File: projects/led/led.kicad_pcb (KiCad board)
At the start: 2 copper layers, 18.2 x 12.8 mm, 3 parts, among them J1 Conn_01x02_Pin

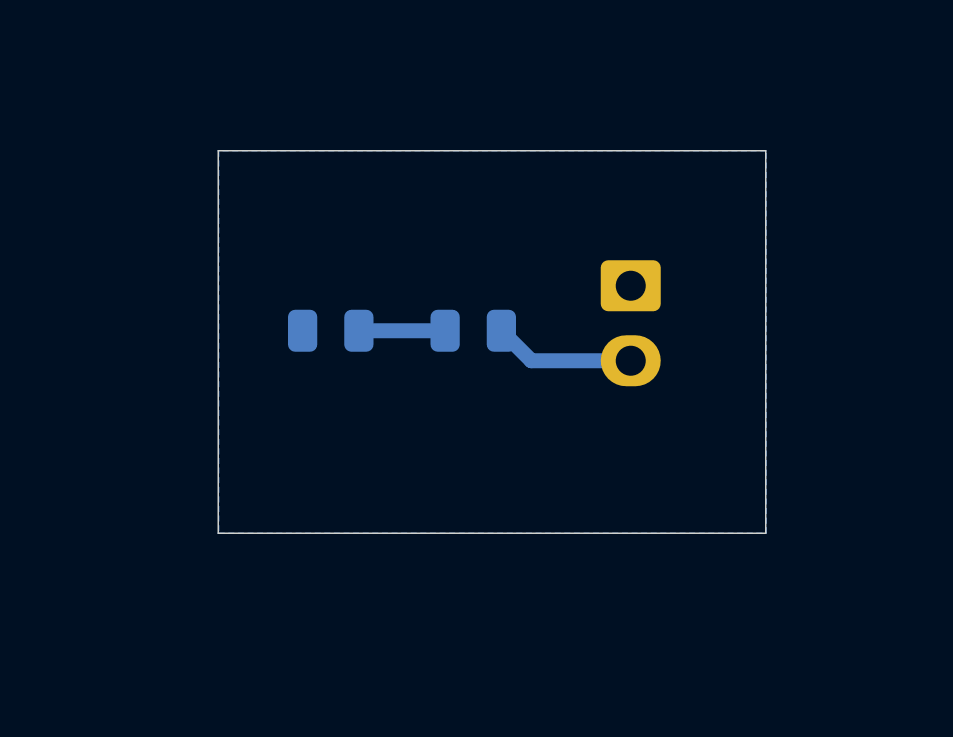
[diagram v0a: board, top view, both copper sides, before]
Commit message: add more
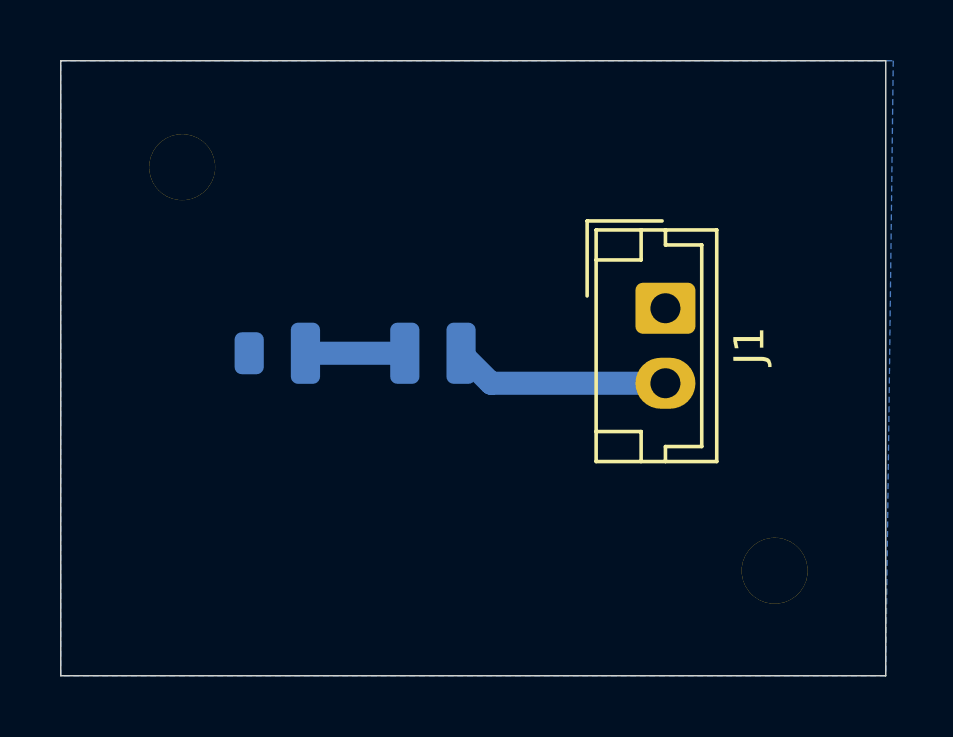
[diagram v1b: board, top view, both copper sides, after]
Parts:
- added H1: MountingHole, MountingHole:MountingHole_2.2mm_M2_DIN965, B.Cu at (118.8, 63.0)
- added H2: MountingHole, MountingHole:MountingHole_2.2mm_M2_DIN965, B.Cu at (138.5, 76.5)
- J1: moved to F.Cu
- moved D1 1.93 mm to (122.0, 69.2)
- moved R1 1.54 mm to (127.2, 69.2)
- moved J1 1.38 mm to (134.9, 67.8)
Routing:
- net VCC: track 4.73 -> 7.23 mm
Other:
- board size 18.2 x 12.8 mm -> 27.5 x 20.5 mm
